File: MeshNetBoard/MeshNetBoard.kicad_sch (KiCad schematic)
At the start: 40 parts, among them J2 Conn_01x02, J3 Micro_SD_Card_Det_Hirose_DM3AT, Q1 Q_PMOS_GSD, SW1 SW_Push, SW2 SW_SPST, U1 XIAO-ESP32-S3-DIP, U2 TPS631000DRLR, U4 MAX9031AU, U5 MCP73831-2-OT

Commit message: maybe doen again...
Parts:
- H1, H2, H3: footprint (none) -> MountingHole:MountingHole_2.2mm_M2_Pad_TopBottom
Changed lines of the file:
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@@
 			)
 		)
-		(property "Footprint" ""
+		(property "Footprint" "MountingHole:MountingHole_2.2mm_M2_Pad_TopBottom"
 			(at 181.61 132.08 0)
 			(hide yes)
@@
 			)
 		)
-		(property "Footprint" ""
+		(property "Footprint" "MountingHole:MountingHole_2.2mm_M2_Pad_TopBottom"
 			(at 210.82 132.08 0)
 			(hide yes)
@@
 			)
 		)
-		(property "Footprint" ""
+		(property "Footprint" "MountingHole:MountingHole_2.2mm_M2_Pad_TopBottom"
 			(at 237.49 132.08 0)
 			(hide yes)

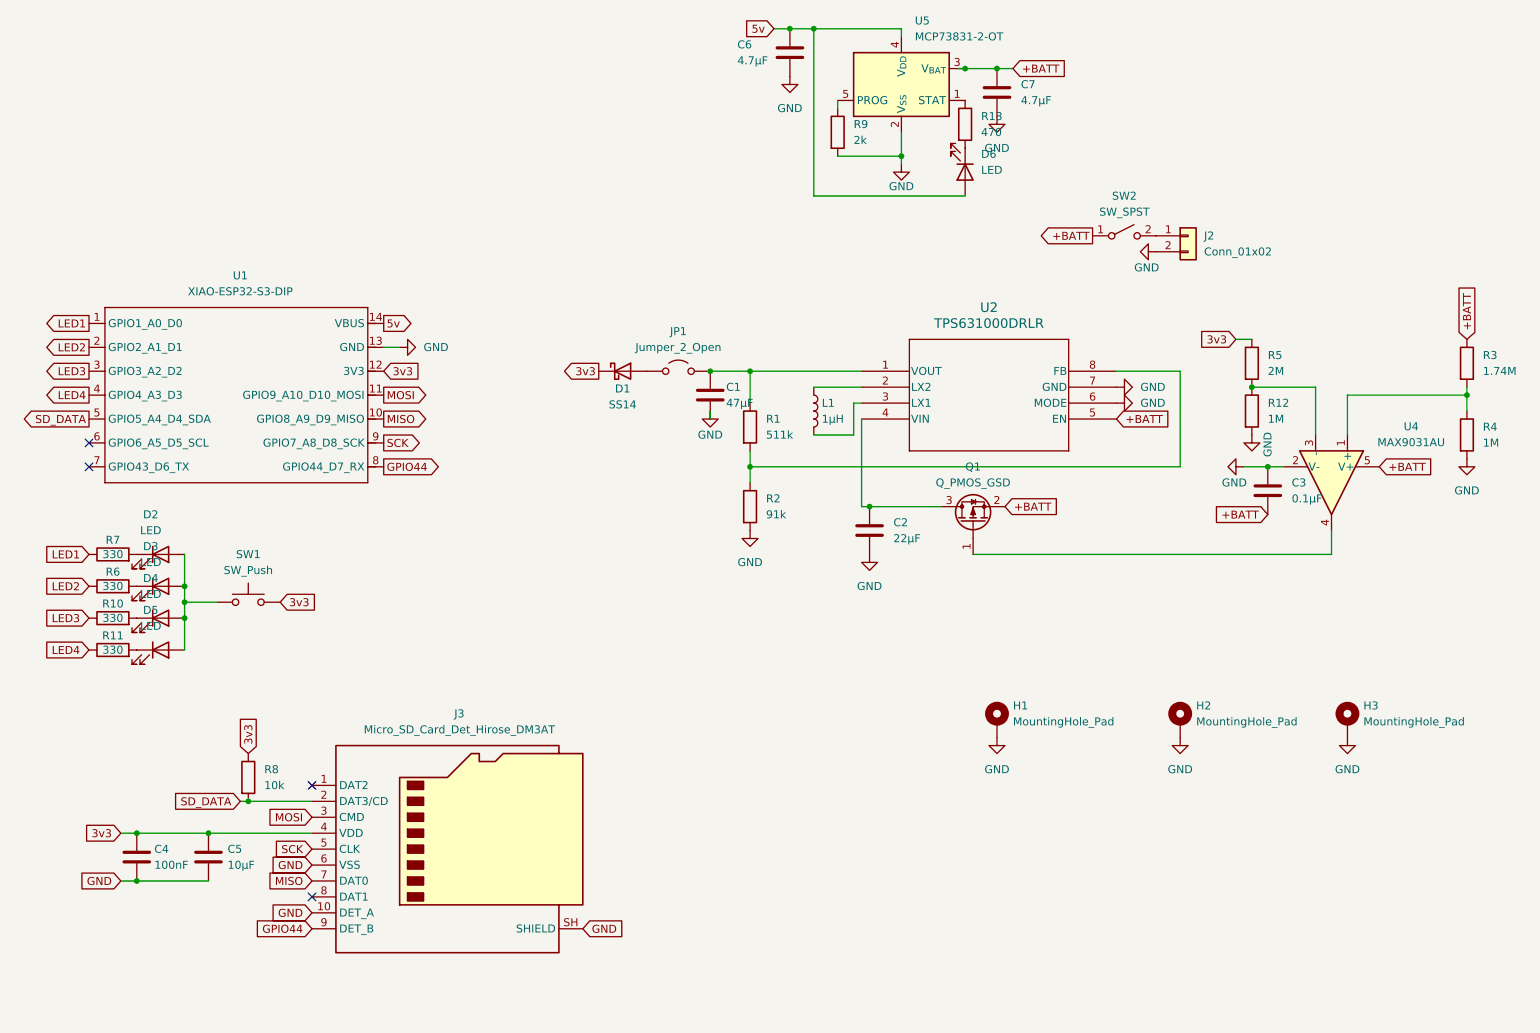
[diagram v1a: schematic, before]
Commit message: resolved stuff
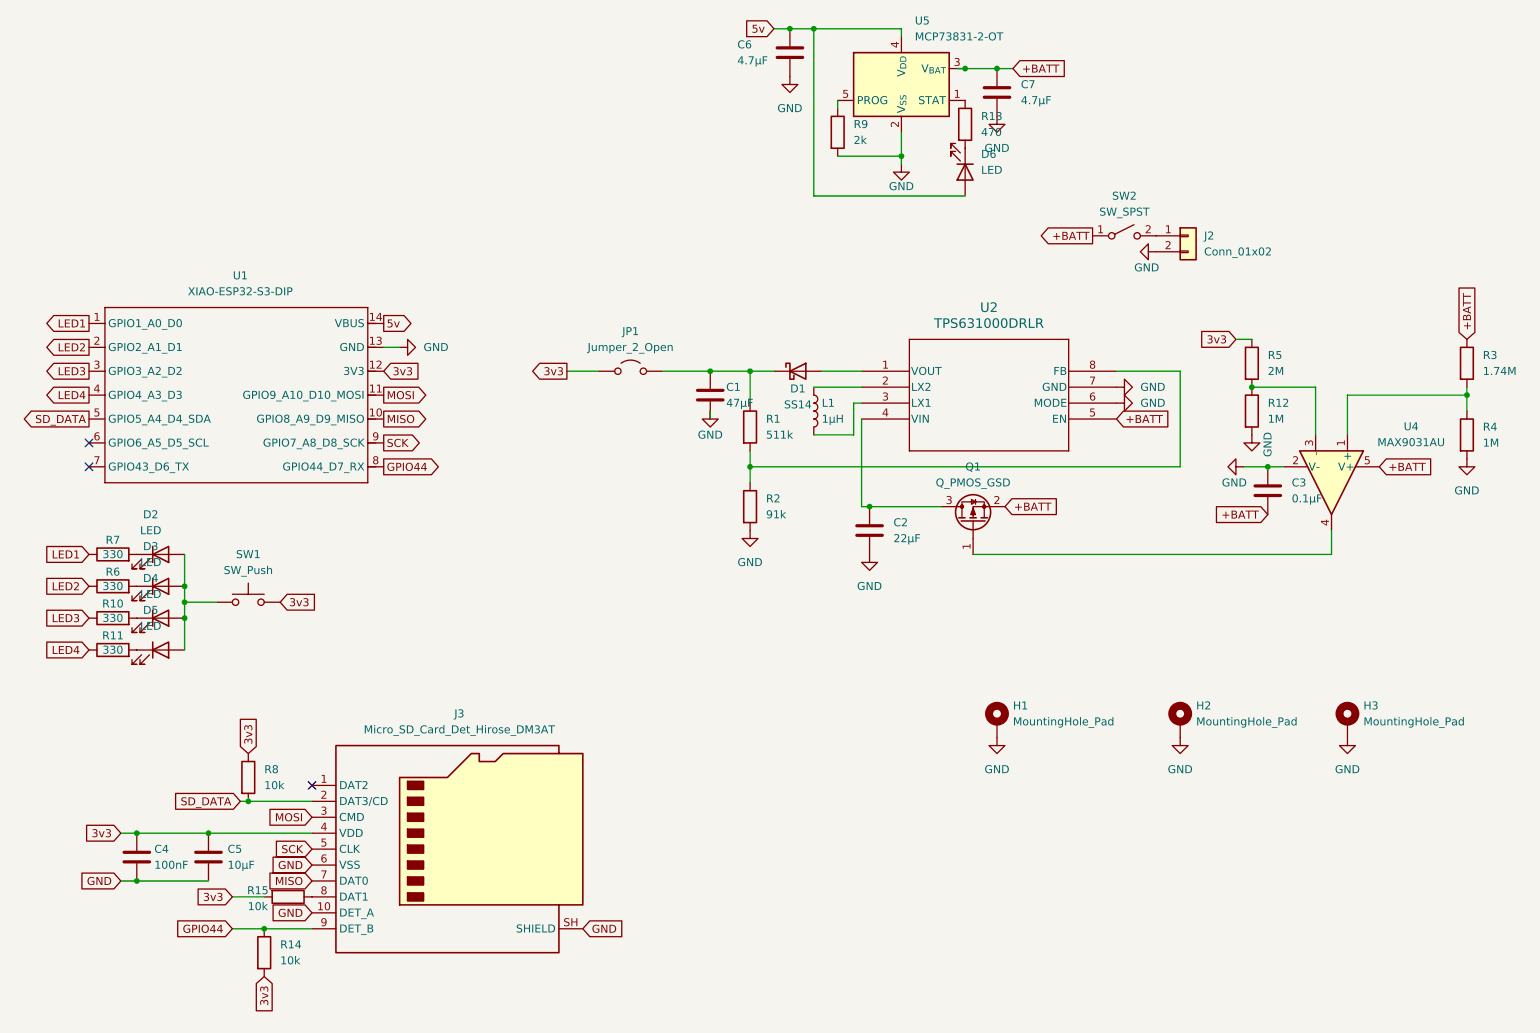
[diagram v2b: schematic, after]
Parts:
- added R14, R15: 10k, Resistor_SMD:R_0603_1608Metric_Pad0.98x0.95mm_HandSolder, symbol Device:R
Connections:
- net 3v3: now also JP1.1 (A), R14.2, R15.2; no longer D1.1 (K)
- net GPIO44: now also R14.1
- net at D1.2 (A): now also U2.1 (VOUT); no longer JP1.1 (A)
- net at C1.1, JP1.2 (B), R1.1: now also D1.1 (K); no longer U2.1 (VOUT)
- net at J3.8 (DAT1): now also R15.1
- no-connect marks 4 -> 3
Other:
- moved on the sheet: D1, JP1
